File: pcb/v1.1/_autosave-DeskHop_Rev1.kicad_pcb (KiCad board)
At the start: 2 copper layers, 66.9 x 74.5 mm, 20 parts, among them J1 Keyboard In, J2 Debug2, J3 Debug1, J4 Mouse In, U2 Pico Primary Custom, U3 TPD4E1U06DBVR, U4 ADuM1201BR, U5 TPD4E1U06DBVR, U6 Pico Primary Custom

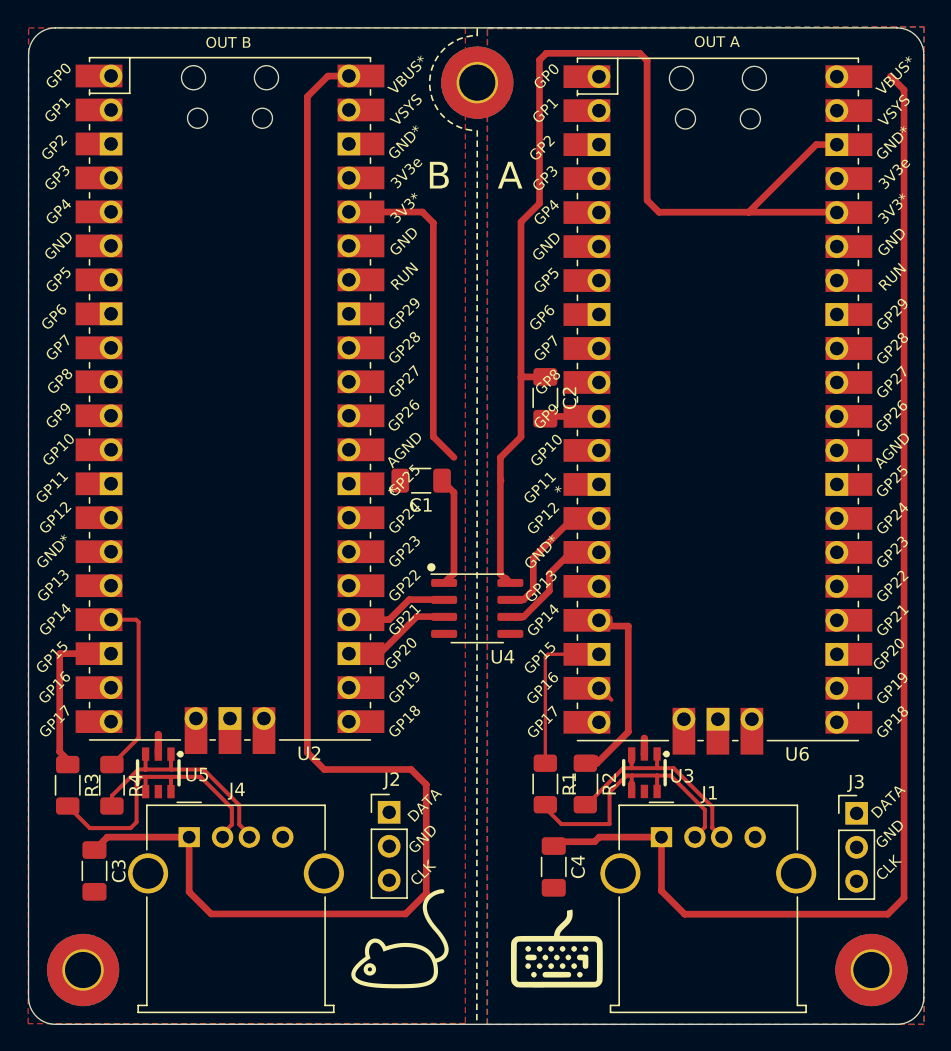
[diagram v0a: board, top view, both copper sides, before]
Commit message: initial rework, connection to be reviewed
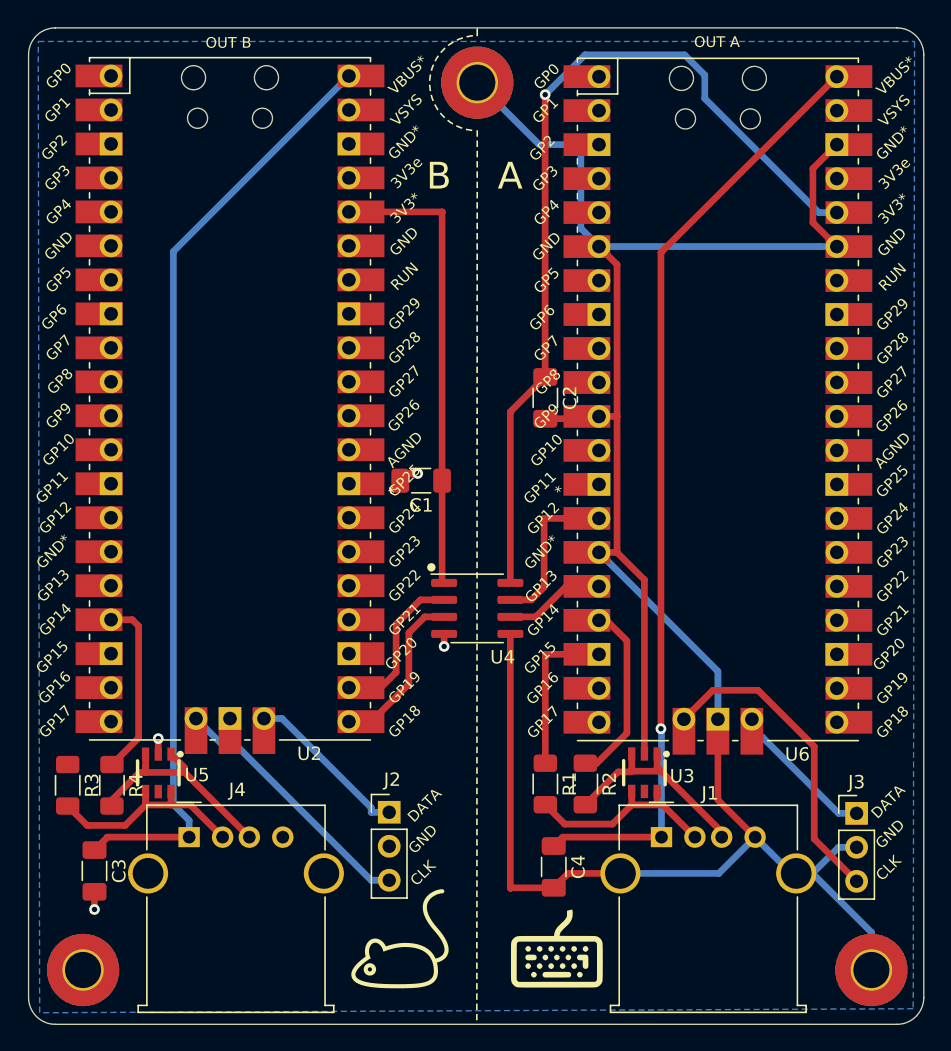
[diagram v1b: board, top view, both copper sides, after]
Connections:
- J2 pad 1: unconnected-(J2-Pin_1-Pad1) -> Net-(J2-Pin_1)
- J2 pad 3: unconnected-(J2-Pin_3-Pad3) -> Net-(J2-Pin_3)
- J3 pad 1: unconnected-(J3-Pin_1-Pad1) -> Net-(J3-Pin_1)
- J3 pad 3: unconnected-(J3-Pin_3-Pad3) -> Net-(J3-Pin_3)
- U2 pad 1: GND -> unconnected-(U2-GPIO0-Pad1)
- U2 pad 11: GND -> unconnected-(U2-GPIO9-Pad11)
- U2 pad 15: unconnected-(U2-GND-Pad15) -> GND
- U2 pad 16: GND -> unconnected-(U2-GPIO13-Pad16)
- U2 pad 21: unconnected-(U2-GPIO18-Pad21) -> UART B TX
- U2 pad 22: unconnected-(U2-GPIO19-Pad22) -> UART B RX
- U2 pad 23: UART B TX -> unconnected-(U2-GPIO20-Pad23)
- U2 pad 24: UART B RX -> unconnected-(U2-GPIO21-Pad24)
- U2 pad 30: GND -> unconnected-(U2-GPIO26-Pad30)
- U2 pad 35: unconnected-(U2-GND-Pad35) -> GND
- U2 pad 36: unconnected-(U2-3V3-Pad36) -> 3V3_BUS2
- U2 pad 38: 3V3_BUS2 -> unconnected-(U2-GND-Pad38)
- U2 pad 40: GND -> VBUS2
- U2 pad 41: unconnected-(U2-SWCLK-Pad41) -> Net-(J2-Pin_3)
- U2 pad 42: unconnected-(U2-GND-Pad42) -> GND
- U2 pad 43: unconnected-(U2-SWDIO-Pad43) -> Net-(J2-Pin_1)
- U6 pad 1: GND2 -> unconnected-(U6-GPIO0-Pad1)
- U6 pad 15: UART A RX -> GND2
- U6 pad 16: GND2 -> UART A RX
- U6 pad 2: GND2 -> unconnected-(U6-GPIO1-Pad2)
- U6 pad 21: GND2 -> unconnected-(U6-GPIO18-Pad21)
- U6 pad 25: GND2 -> unconnected-(U6-GPIO22-Pad25)
- U6 pad 3: unconnected-(U6-GPIO2-Pad3) -> GND2
- U6 pad 30: GND2 -> unconnected-(U6-GPIO26-Pad30)
- U6 pad 35: unconnected-(U6-GND-Pad35) -> GND2
- U6 pad 36: unconnected-(U6-3V3-Pad36) -> Net-(U4-VDD2)
- U6 pad 38: Net-(U4-VDD2) -> GND2
- U6 pad 40: GND2 -> VBUS1
- U6 pad 41: unconnected-(U6-SWCLK-Pad41) -> Net-(J3-Pin_3)
- U6 pad 42: unconnected-(U6-GND-Pad42) -> GND2
- U6 pad 43: unconnected-(U6-SWDIO-Pad43) -> Net-(J3-Pin_1)
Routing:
- net GND2: track 7.67 -> 175.8 mm
- net VBUS2: track 101.4 -> 70.3 mm
- net 3V3_BUS2: track 8.82 -> 34.8 mm
- net unconnected-(U2-3V3-Pad36): track 24.8 -> 0.00 mm
- net Net-(J3-Pin_3): track 0.00 -> 23.8 mm
- net VBUS1: track 93.5 -> 70.6 mm, vias 0 -> 1
- net Net-(J2-Pin_3): track 0.00 -> 19.4 mm
- net Net-(U4-VDD2): track 85.2 -> 66.5 mm, vias 0 -> 1
- net Net-(U2-GPIO15): track 12.5 -> 0.00 mm
- net Net-(J2-Pin_1): track 0.00 -> 12.5 mm
- net Net-(J3-Pin_1): track 0.00 -> 11.5 mm
- net OA-: track 22.0 -> 15.4 mm
- net OB-: track 22.0 -> 15.8 mm
- net UART B TX: track 8.36 -> 12.6 mm
- net UART B RX: track 7.83 -> 11.9 mm
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- added copper zone on B.Cu, net GND
- removed copper zone on F.Cu, net GND
- removed copper zone on B.Cu, net GND2
- removed copper zone on F.Cu, net GND2
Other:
- board text removed: "${REFERENCE}"
